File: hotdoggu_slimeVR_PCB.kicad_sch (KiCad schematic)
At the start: 8 parts, among them J1 Conn_01x04_Pin, J2 Conn_01x02_Pin, SW1 SW_SPDT_312, U2 module_mpu6050

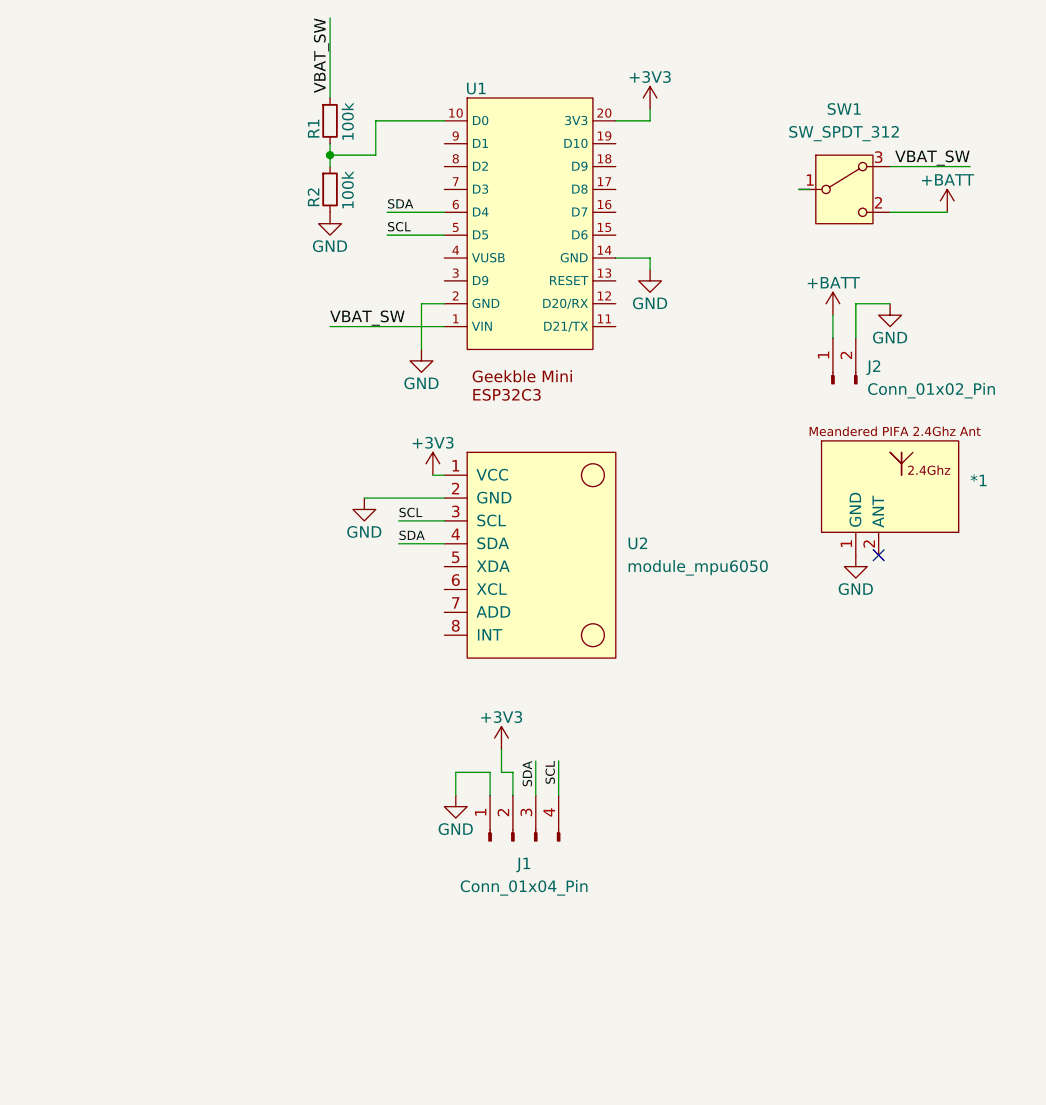
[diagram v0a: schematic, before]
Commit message: pattern, sym, footprint update
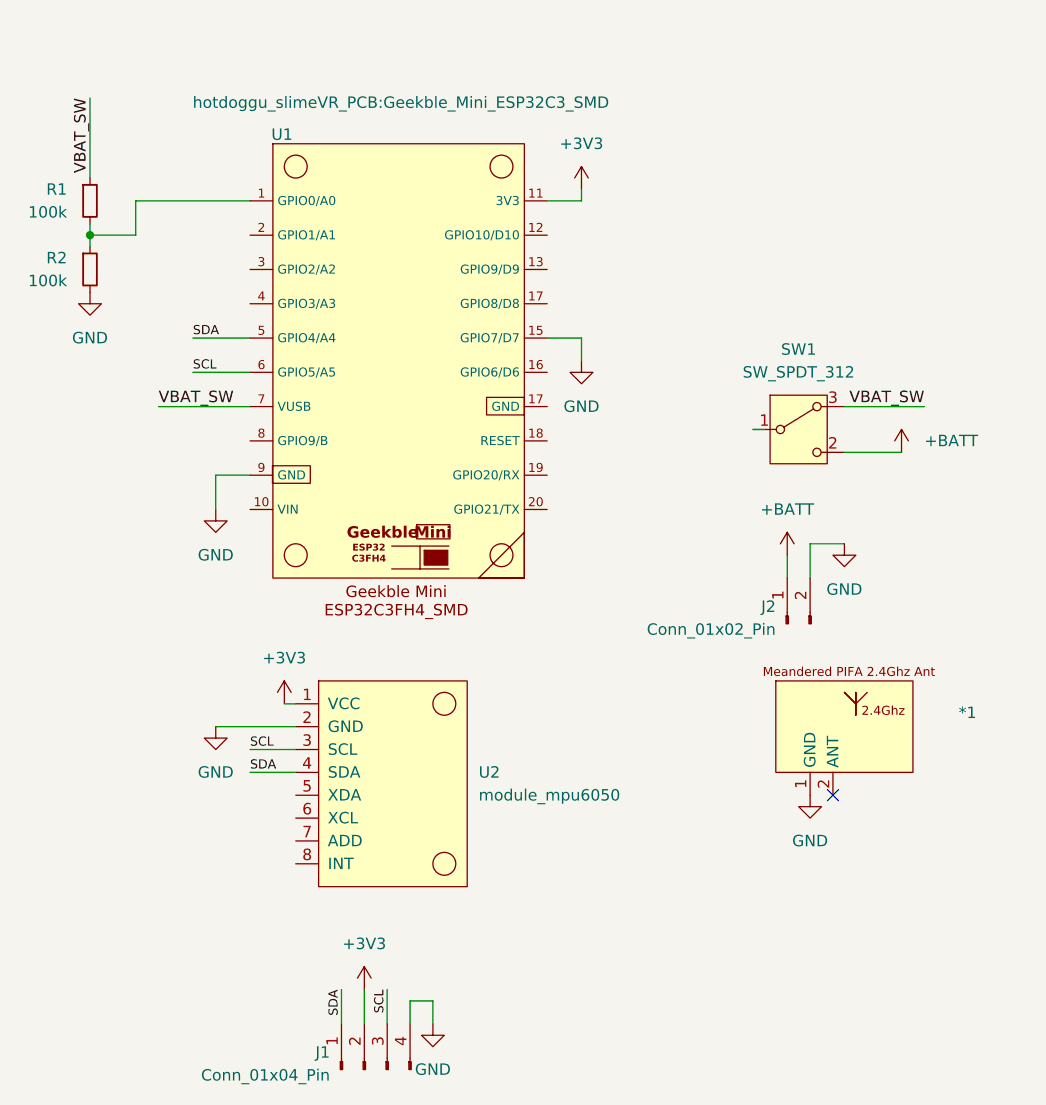
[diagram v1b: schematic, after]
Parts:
- U1: footprint hotdoggu_slimeVR_PCB:Geekble_Mini_ESP32C3 -> hotdoggu_slimeVR_PCB:Geekble_Mini_ESP32C3_SMD; symbol hotdoggu_slimeVR_PCB:Geekble_Mini_ESP32C3 -> hotdoggu_slimeVR_PCB:Geekble_Mini_ESP32C3FH4_SMD
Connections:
- net +3V3: now also U1.11 (3V3); no longer U1.20 (3V3)
- net GND: now also J1.4 (Pin_4), U1.15 (GPIO7/D7), U1.9 (GND); no longer J1.1 (Pin_1), U1.14 (GND), U1.2 (GND)
- net SCL: now also J1.3 (Pin_3), U1.6 (GPIO5/A5); no longer J1.4 (Pin_4), U1.5 (D5)
- net SDA: now also J1.1 (Pin_1), U1.5 (GPIO4/A4); no longer J1.3 (Pin_3), U1.6 (D4)
- net VBAT_SW: now also U1.7 (VUSB); no longer U1.1 (VIN)
- net at R1.2, R2.1: now also U1.1 (GPIO0/A0); no longer U1.10 (D0)
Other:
- moved on the sheet: *1, J1, J2, R1, R2, SW1, U2
